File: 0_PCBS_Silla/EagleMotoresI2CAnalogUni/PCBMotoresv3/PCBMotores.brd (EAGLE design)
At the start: 100 x 50.3 mm, 41 parts, among them IC1 MEGA8-AI, IC2 REG1117, Q2 2SC3838T146

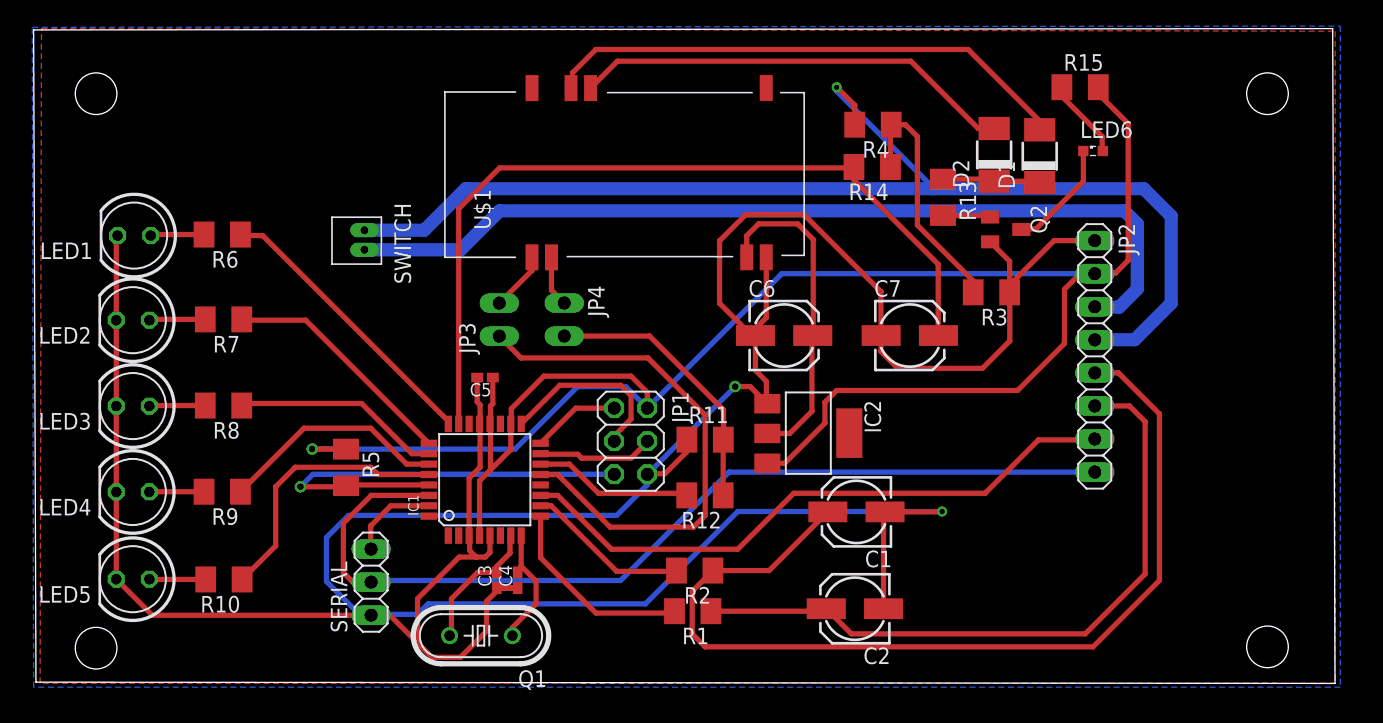
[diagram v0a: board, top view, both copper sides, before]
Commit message: 13 marzo 2020
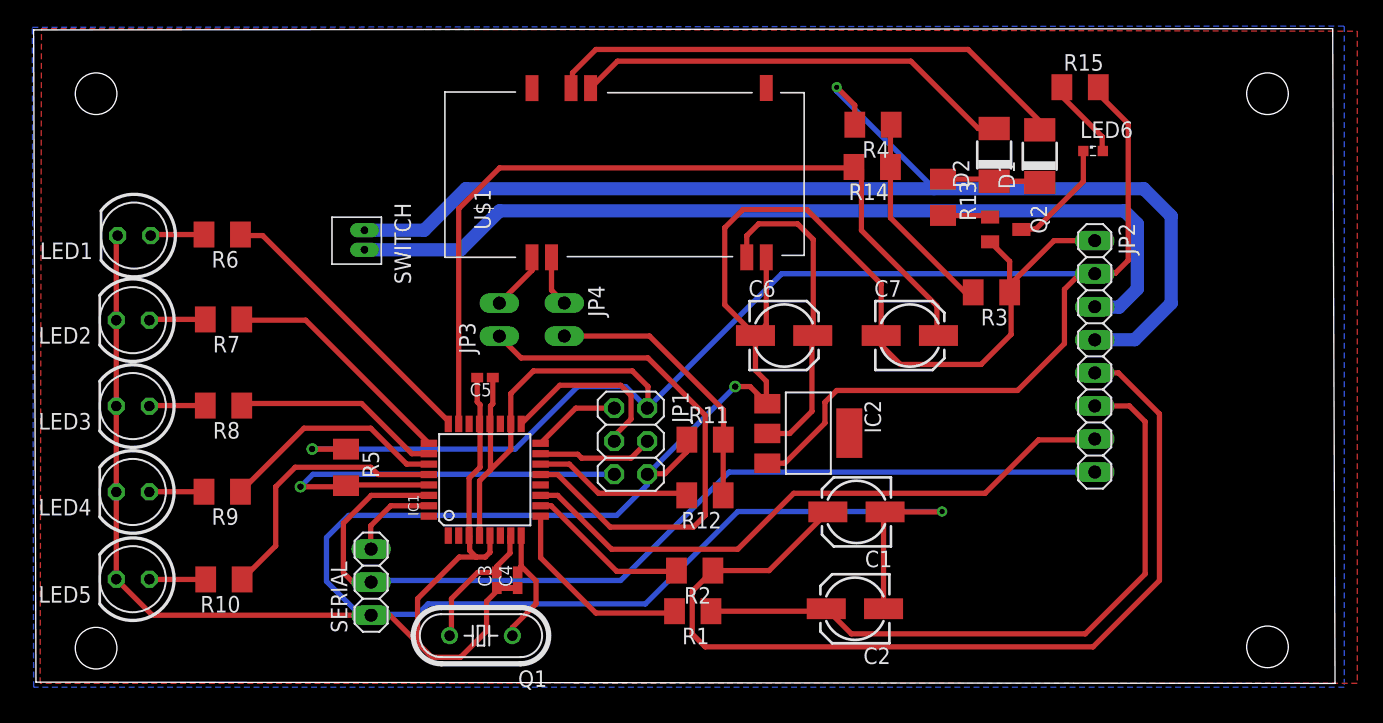
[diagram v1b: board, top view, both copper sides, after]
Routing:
- net N$26: track 19.4 -> 15.9 mm
- net 5V: track 152.7 -> 154.1 mm
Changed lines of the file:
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@@
 <wire x1="56.5" y1="22.9" x2="56.5" y2="21.251" width="0.4064" layer="1"/>
 <wire x1="56.5" y1="21.251" x2="56.5704" y2="21.1806" width="0.4064" layer="1"/>
-<wire x1="56.49" y1="32.43" x2="56.49" y2="27.79" width="0.4064" layer="1"/>
-<wire x1="56.49" y1="27.79" x2="55.7" y2="27" width="0.4064" layer="1"/>
-<wire x1="55.7" y1="27" x2="55.7" y2="26.46" width="0.4064" layer="1"/>
-<wire x1="55.7" y1="26.46" x2="55.66" y2="26.42" width="0.4064" layer="1"/>
 <wire x1="65.5" y1="5.43" x2="65.5" y2="12.75" width="0.4064" layer="1"/>
 <wire x1="65.5" y1="12.75" x2="65.62" y2="12.87" width="0.4064" layer="1"/>
-<wire x1="55.7" y1="27" x2="55.6" y2="26.9" width="0.4064" layer="1"/>
-<wire x1="55.6" y1="26.9" x2="54.9" y2="26.9" width="0.4064" layer="1"/>
-<wire x1="54.9" y1="26.9" x2="52.9" y2="28.9" width="0.4064" layer="1"/>
-<wire x1="52.9" y1="28.9" x2="52.9" y2="33.7" width="0.4064" layer="1"/>
-<wire x1="52.9" y1="33.7" x2="54.9" y2="35.7" width="0.4064" layer="1"/>
-<wire x1="54.9" y1="35.7" x2="59.4" y2="35.7" width="0.4064" layer="1"/>
-<wire x1="59.4" y1="35.7" x2="65.3" y2="29.8" width="0.4064" layer="1"/>
-<wire x1="65.3" y1="29.8" x2="65.3" y2="26.44" width="0.4064" layer="1"/>
-<wire x1="65.3" y1="26.44" x2="65.32" y2="26.42" width="0.4064" layer="1"/>
 <wire x1="47.35" y1="15.76" x2="47.35" y2="14.95" width="0.4064" layer="16"/>
 <wire x1="47.35" y1="14.95" x2="45" y2="12.6" width="0.4064" layer="16"/>
@@
 <wire x1="29.7" y1="5" x2="26.2" y2="5" width="0.4064" layer="16"/>
 <wire x1="26.2" y1="5" x2="26.13" y2="4.93" width="0.4064" layer="16"/>
-<wire x1="65.3" y1="26.44" x2="65.3" y2="25.2" width="0.4064" layer="1"/>
-<wire x1="65.3" y1="25.2" x2="66.6" y2="23.9" width="0.4064" layer="1"/>
-<wire x1="66.6" y1="23.9" x2="73.1" y2="23.9" width="0.4064" layer="1"/>
-<wire x1="73.1" y1="23.9" x2="75.2" y2="26" width="0.4064" layer="1"/>
-<wire x1="75.2" y1="26" x2="75.2" y2="29.73" width="0.4064" layer="1"/>
-<wire x1="75.2" y1="29.73" x2="75.19" y2="29.74" width="0.4064" layer="1"/>
 <wire x1="75.19" y1="29.74" x2="75.19" y2="30.3" width="0.4064" layer="1"/>
 <wire x1="75.19" y1="30.3" x2="75.19" y2="32.12" width="0.4064" layer="1"/>
@@
 <polygon width="0.4064" layer="16" isolate="1">
 <vertex x="0.1" y="50.1"/>
-<vertex x="100.6" y="50.2"/>
-<vertex x="100.6" y="-0.6"/>
+<vertex x="100.9" y="50.2"/>
+<vertex x="100.9" y="-0.6"/>
 <vertex x="0.2" y="-0.6"/>
 </polygon>
 <polygon width="0.4064" layer="1" isolate="1">
 <vertex x="0.8" y="50"/>
-<vertex x="100.2" y="49.8"/>
-<vertex x="100.2" y="-0.3"/>
+<vertex x="101.9" y="49.8"/>
+<vertex x="101.9" y="-0.3"/>
 <vertex x="0.7" y="-0.3"/>
 </polygon>
+<wire x1="56.49" y1="32.43" x2="56.49" y2="27.25" width="0.4064" layer="1"/>
+<wire x1="56.49" y1="27.25" x2="55.66" y2="26.42" width="0.4064" layer="1"/>
+<wire x1="65.32" y1="26.42" x2="65.32" y2="30.38" width="0.4064" layer="1"/>
+<wire x1="65.32" y1="30.38" x2="59.6" y2="36.1" width="0.4064" layer="1"/>
+<wire x1="59.6" y1="36.1" x2="54.7" y2="36.1" width="0.4064" layer="1"/>
+<wire x1="54.7" y1="36.1" x2="53.3" y2="34.7" width="0.4064" layer="1"/>
+<wire x1="53.3" y1="34.7" x2="53.3" y2="28.78" width="0.4064" layer="1"/>
+<wire x1="53.3" y1="28.78" x2="55.66" y2="26.42" width="0.4064" layer="1"/>
+<wire x1="65.32" y1="26.42" x2="65.32" y2="25.68" width="0.4064" layer="1"/>
+<wire x1="65.32" y1="25.68" x2="66.8" y2="24.2" width="0.4064" layer="1"/>
+<wire x1="66.8" y1="24.2" x2="73" y2="24.2" width="0.4064" layer="1"/>
+<wire x1="73" y1="24.2" x2="75.3" y2="26.5" width="0.4064" layer="1"/>
+<wire x1="75.3" y1="26.5" x2="75.3" y2="29.63" width="0.4064" layer="1"/>
+<wire x1="75.3" y1="29.63" x2="75.19" y2="29.74" width="0.4064" layer="1"/>
 </signal>
 <signal name="RX">
@@
 <wire x1="36.86" y1="19.6326" x2="36.86" y2="17.66" width="0.4064" layer="1"/>
 <wire x1="36.86" y1="17.66" x2="35.3" y2="16.1" width="0.4064" layer="1"/>
-<wire x1="47.35" y1="20.84" x2="47.35" y2="22.05" width="0.4064" layer="1"/>
-<wire x1="47.35" y1="22.05" x2="46.1" y2="23.3" width="0.4064" layer="1"/>
-<wire x1="46.1" y1="23.3" x2="39.4" y2="23.3" width="0.4064" layer="1"/>
-<wire x1="39.4" y1="23.3" x2="36.9" y2="20.8" width="0.4064" layer="1"/>
-<wire x1="36.9" y1="20.8" x2="36.9" y2="19.6726" width="0.4064" layer="1"/>
-<wire x1="36.9" y1="19.6726" x2="36.86" y2="19.6326" width="0.4064" layer="1"/>
 <wire x1="35.48" y1="23.19" x2="35.48" y2="21.18" width="0.4064" layer="1"/>
 <wire x1="35.48" y1="21.18" x2="35.3" y2="21" width="0.4064" layer="1"/>
@@
 <wire x1="83.3" y1="31.2" x2="81.76" y2="31.2" width="0.4064" layer="1"/>
 <wire x1="81.76" y1="31.2" x2="81.73" y2="31.17" width="0.4064" layer="1"/>
+<wire x1="36.86" y1="19.6326" x2="36.86" y2="21.96" width="0.4064" layer="1"/>
+<wire x1="36.86" y1="21.96" x2="38.6" y2="23.7" width="0.4064" layer="1"/>
+<wire x1="38.6" y1="23.7" x2="46.2" y2="23.7" width="0.4064" layer="1"/>
+<wire x1="46.2" y1="23.7" x2="47.4" y2="22.5" width="0.4064" layer="1"/>
+<wire x1="47.4" y1="22.5" x2="47.4" y2="20.89" width="0.4064" layer="1"/>
+<wire x1="47.4" y1="20.89" x2="47.35" y2="20.84" width="0.4064" layer="1"/>
 </signal>
 <signal name="FRENOS">
@@
 <wire x1="63.8" y1="39.2" x2="63.4" y2="39.2" width="0.4064" layer="1"/>
 <wire x1="63.4" y1="39.2" x2="63.23" y2="39.37" width="0.4064" layer="1"/>
-<wire x1="63.23" y1="39.37" x2="63.23" y2="38.37" width="0.4064" layer="1"/>
-<wire x1="63.23" y1="38.37" x2="69.7" y2="31.9" width="0.4064" layer="1"/>
-<wire x1="69.7" y1="31.9" x2="69.7" y2="26.44" width="0.4064" layer="1"/>
-<wire x1="69.7" y1="26.44" x2="69.72" y2="26.42" width="0.4064" layer="1"/>
+<wire x1="63.8" y1="39.2" x2="63.8" y2="34.5" width="0.4064" layer="1"/>
+<wire x1="63.8" y1="34.5" x2="69.6" y2="28.7" width="0.4064" layer="1"/>
+<wire x1="69.6" y1="28.7" x2="69.6" y2="26.54" width="0.4064" layer="1"/>
+<wire x1="69.6" y1="26.54" x2="69.72" y2="26.42" width="0.4064" layer="1"/>
 </signal>
 <signal name="N$10">
@@
 <wire x1="66.03" y1="39.37" x2="66.03" y2="42.56" width="0.4064" layer="1"/>
 <wire x1="66.03" y1="42.56" x2="66.09" y2="42.62" width="0.4064" layer="1"/>
-<wire x1="66.09" y1="42.62" x2="67.18" y2="42.62" width="0.4064" layer="1"/>
-<wire x1="67.18" y1="42.62" x2="68.1" y2="41.7" width="0.4064" layer="1"/>
-<wire x1="68.1" y1="41.7" x2="68.1" y2="34.9" width="0.4064" layer="1"/>
-<wire x1="68.1" y1="34.9" x2="72.4" y2="30.6" width="0.4064" layer="1"/>
-<wire x1="72.4" y1="30.6" x2="72.4" y2="29.75" width="0.4064" layer="1"/>
-<wire x1="72.4" y1="29.75" x2="72.39" y2="29.74" width="0.4064" layer="1"/>
+<wire x1="66.03" y1="39.37" x2="66.03" y2="35.47" width="0.4064" layer="1"/>
+<wire x1="66.03" y1="35.47" x2="71.8" y2="29.7" width="0.4064" layer="1"/>
+<wire x1="71.8" y1="29.7" x2="72.35" y2="29.7" width="0.4064" layer="1"/>
+<wire x1="72.35" y1="29.7" x2="72.39" y2="29.74" width="0.4064" layer="1"/>
 </signal>
 <signal name="N$21">
